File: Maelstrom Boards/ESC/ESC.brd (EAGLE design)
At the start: 101.6 x 101.6 mm, 31 parts, among them P5 MALE1PINHEADER, P6 MALE1PINHEADER, P7 MALE1PINHEADER, P8 MALE1PINHEADER

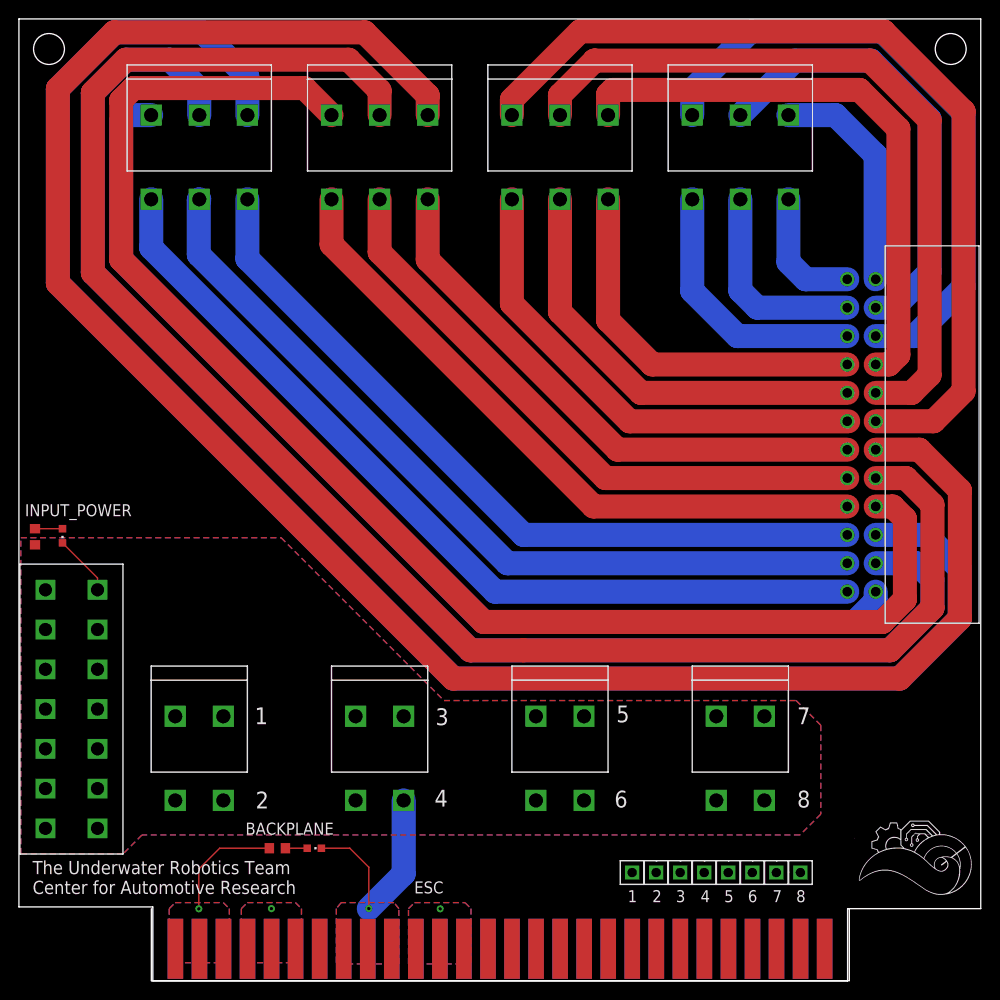
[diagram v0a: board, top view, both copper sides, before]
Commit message: Finished ESC board, need to go back for minor changes.
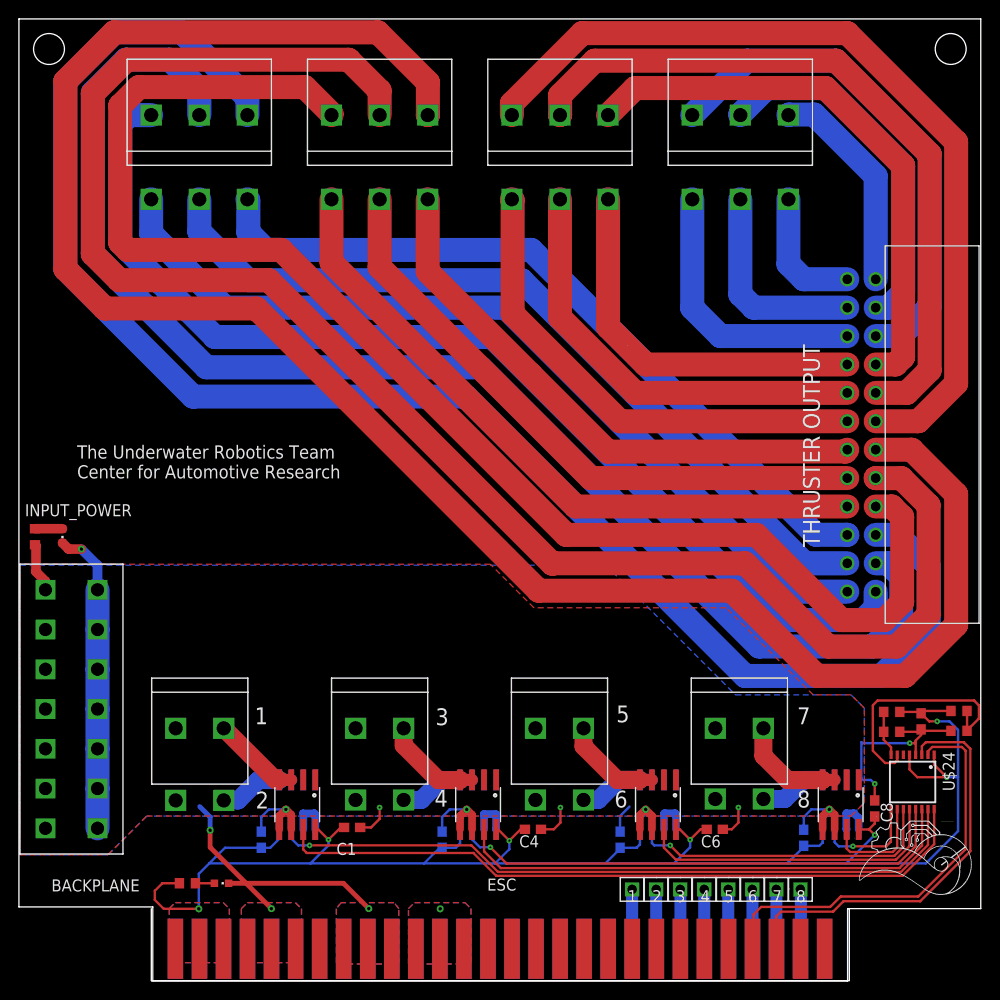
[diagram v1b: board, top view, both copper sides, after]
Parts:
- removed U$2, U$3, U$4, U$5, U$6, U$7, U$8, U$9: 1711725, Screw_Terminals:1711725
- added 1C, 2C, 3C, 4C, 5C, 6C, 7C, 8C: ACS722, ACS722:SOIC-8
- added 1CONNECT, 2CONNECT, 3CONNECT, 4CONNECT, 5CONNECT, 7CONNECT, 8CONNECT, CONNECT: 1711725, Screw_Terminals:1711725
- added C1, C2, C3, C4, C5, C6, C7, C8, C9: (no value), rcl:C0603
- added R3, R4, R5, R6: (no value), resistor:R0603
- added U$24: ADC128D818, ADC128D818:TSSOP-16
- moved 1 57.8 mm to (19.1, 91.4), flipped to the top, turned to 0 degrees
- moved 2 57.8 mm to (19.1, 82.5), flipped to the bottom, turned to 0 degrees
- moved 7 57.8 mm to (76.2, 91.4), flipped to the top, turned to 0 degrees
- moved 8 57.8 mm to (76.2, 82.5), flipped to the bottom, turned to 0 degrees
- moved 3 21.0 mm to (38.1, 91.4), flipped to the top, turned to 0 degrees
- moved 4 21.0 mm to (38.1, 82.5), flipped to the bottom, turned to 0 degrees
- moved 5 21.0 mm to (57.1, 91.4), flipped to the top, turned to 0 degrees
- moved 6 21.0 mm to (57.1, 82.5), flipped to the bottom, turned to 0 degrees
- moved BACKPLANE 10.5 mm to (21.4, 10.3)
- moved R2 10.2 mm to (17.8, 10.3)
- moved P5 1.78 mm to (74.9, 9.65)
- moved P6 1.78 mm to (77.5, 9.65)
- moved P7 1.78 mm to (80.0, 9.65)
- moved P8 1.78 mm to (82.5, 9.65)
- moved U$20 1.78 mm to (64.8, 9.65)
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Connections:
- new net 0ADC: 1C.VIOUT, U$24.IN0
- new net 1ADC: 2C.VIOUT, U$24.IN1
- new net 2ADC: 3C.VIOUT, U$24.IN2
- new net 3ADC: 4C.VIOUT, U$24.IN3
- new net 4ADC: 5C.VIOUT, U$24.IN4
- new net 5ADC: 6C.VIOUT, U$24.IN5
- new net 6ADC: 7C.VIOUT, U$24.IN6
- new net 7ADC: 8C.VIOUT, U$24.IN7
- new net N$30: 1C.IP-1, 1C.IP-2, 1CONNECT.RED
- new net N$32: 2C.IP+1, 2C.IP+2, 2CONNECT.BLACK
- new net N$33: 3C.IP-1, 3C.IP-2, 3CONNECT.RED
- new net N$34: 5C.IP-1, 5C.IP-2, 5CONNECT.RED
- new net N$35: 4C.IP+1, 4C.IP+2, 4CONNECT.BLACK
- new net N$36: 6C.IP+1, 6C.IP+2, CONNECT.BLACK
- new net N$37: 7C.IP-1, 7C.IP-2, 7CONNECT.RED
- new net N$38: 8C.IP+1, 8C.IP+2, 8CONNECT.BLACK
- new net N$44: R3.2, R4.1, U$24.A0
- new net N$46: R5.1, R6.2, U$24.A1
- new net SCL: U$1.31, U$24.SCL
- new net SDA: U$1.32, U$24.SDA
- net +3V3: now also 1C.VCC, 2C.VCC, 3C.VCC, 4C.VCC, 5C.VCC, 6C.VCC, 7C.VCC, 8C.VCC, C1.2, C2.2, C3.2, C4.2, C5.2, C6.2, C7.2, C8.2, C9.1, R3.1, R6.1, U$24.V+, U$24.VREF
- net BALANCED+: now also 1C.IP+1, 1C.IP+2, 2CONNECT.RED, 3C.IP+1, 3C.IP+2, 4CONNECT.RED, 5C.IP+1, 5C.IP+2, 7C.IP+1, 7C.IP+2, 8CONNECT.RED, CONNECT.RED; no longer U$2.RED, U$3.RED, U$4.RED, U$5.RED, U$6.RED, U$7.RED, U$8.RED, U$9.RED
- net GND: now also 1C.BW_SEL, 1C.GND, 1CONNECT.BLACK, 2C.BW_SEL, 2C.GND, 2C.IP-1, 2C.IP-2, 3C.BW_SEL, 3C.GND, 3CONNECT.BLACK, 4C.BW_SEL, 4C.GND, 4C.IP-1, 4C.IP-2, 5C.BW_SEL, 5C.GND, 5CONNECT.BLACK, 6C.BW_SEL, 6C.GND, 6C.IP-1, 6C.IP-2, 7C.BW_SEL, 7C.GND, 7CONNECT.BLACK, 8C.BW_SEL, 8C.GND, 8C.IP-1, 8C.IP-2, C1.1, C2.1, C3.1, C4.1, C5.1, C6.1, C7.1, C8.1, C9.2, R4.2, R5.2, U$24.GND; no longer U$2.BLACK, U$3.BLACK, U$4.BLACK, U$5.BLACK, U$6.BLACK, U$7.BLACK, U$8.BLACK, U$9.BLACK
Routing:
- net +3V3: track 12.6 -> 182.9 mm, vias 1 -> 7
- net N$4: track 179.8 -> 13.7 mm
- net N$9: track 206.3 -> 40.4 mm
- net N$17: track 40.0 -> 204.3 mm
- net N$22: track 13.6 -> 170.5 mm
- net N$8: track 179.8 -> 46.1 mm
- net N$18: track 45.8 -> 177.9 mm
- net N$3: track 152.5 -> 21.9 mm
- net N$1: track 21.7 -> 145.2 mm
- net GND: track 29.6 -> 149.1 mm, vias 2 -> 13
- net N$7: track 152.5 -> 52.2 mm
- net N$16: track 51.7 -> 151.0 mm
- net N$24: track 28.0 -> 114.7 mm
- net N$2: track 115.5 -> 29.1 mm
- net 0ADC: track 0.00 -> 75.0 mm
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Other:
- board text added: "THRUSTER OUTPUT"
